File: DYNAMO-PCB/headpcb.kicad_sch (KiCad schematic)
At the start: 15 parts, among them J10 Conn_01x03_Pin, J11 Conn_01x03_Pin, J12 Conn_01x03_Pin, J33 Conn_02x05_Counter_Clockwise, J5 Conn_01x02_Pin, J6 Conn_01x03_Pin, J7 Conn_01x08_Socket, J8 Conn_01x03_Pin, J9 Conn_01x03_Pin

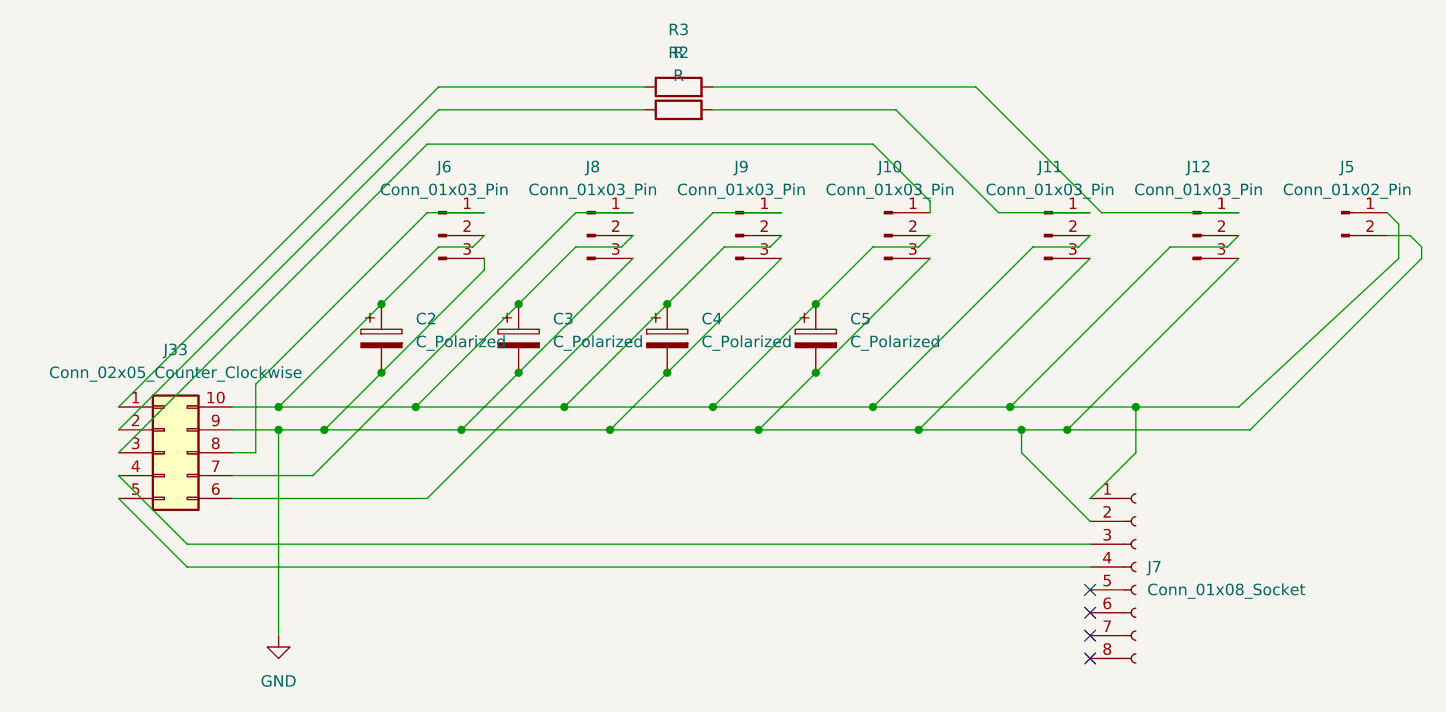
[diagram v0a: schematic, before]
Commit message: schematic wip
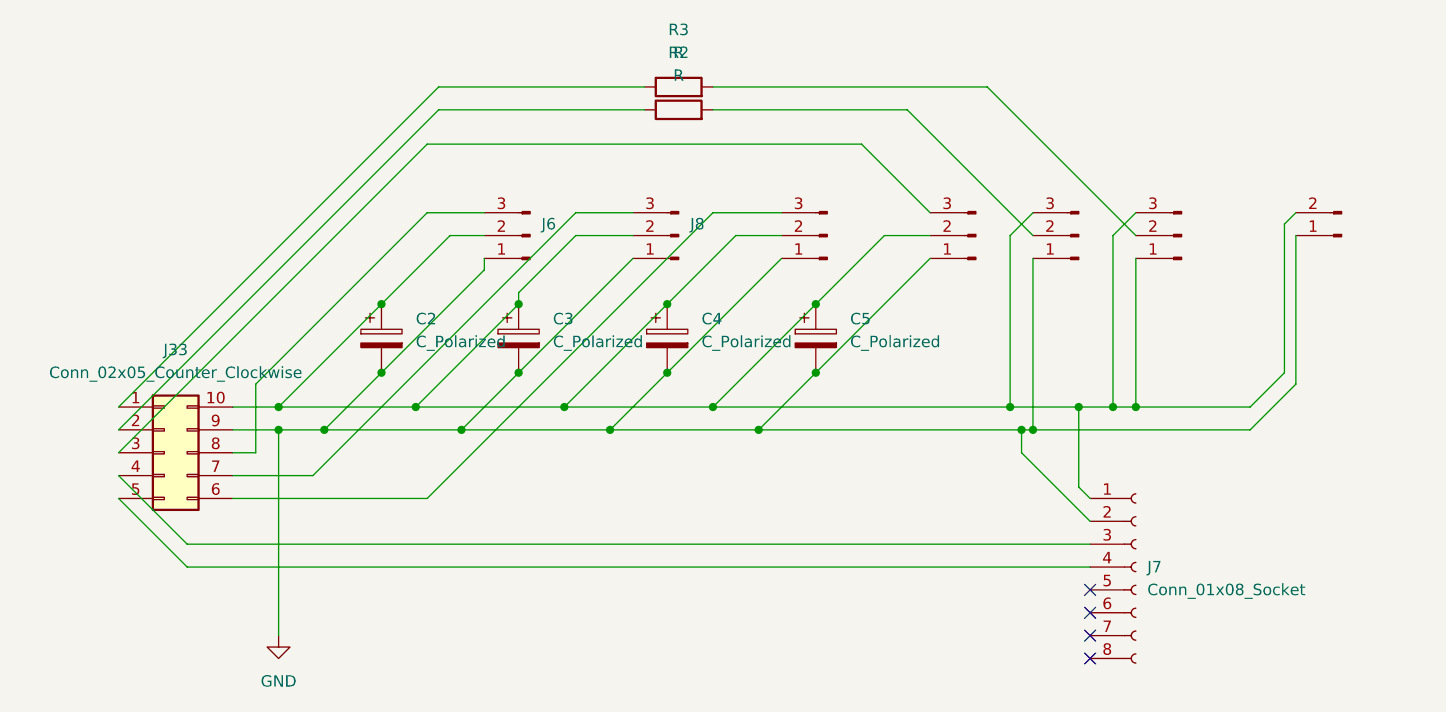
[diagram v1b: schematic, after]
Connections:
- net GND: now also J10.1 (Pin_1), J11.1 (Pin_1), J5.1 (Pin_1), J6.1 (Pin_1), J8.1 (Pin_1), J9.1 (Pin_1); no longer J10.3 (Pin_3), J11.3 (Pin_3), J12.3 (Pin_3), J5.2 (Pin_2), J6.3 (Pin_3), J8.3 (Pin_3), J9.3 (Pin_3)
- net at C2.1, C3.1, C4.1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: now also J11.3 (Pin_3), J12.1 (Pin_1), J12.3 (Pin_3), J5.2 (Pin_2); no longer J11.2 (Pin_2), J12.2 (Pin_2), J5.1 (Pin_1)
- net at R3.2: now also J12.2 (Pin_2); no longer J12.1 (Pin_1)
- net at J33.3 (Pin_3): now also J10.3 (Pin_3); no longer J10.1 (Pin_1)
- net at R2.2: now also J11.2 (Pin_2); no longer J11.1 (Pin_1)
- net at J33.6 (Pin_6): now also J9.3 (Pin_3); no longer J9.1 (Pin_1)
- net at J33.7 (Pin_7): now also J8.3 (Pin_3); no longer J8.1 (Pin_1)
- net at J33.8 (Pin_8): now also J6.3 (Pin_3); no longer J6.1 (Pin_1)
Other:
- moved on the sheet: J6, J8
